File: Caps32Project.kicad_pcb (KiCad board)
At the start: 2 copper layers, 23.9 x 20.7 mm, 41 parts, among them J1 Sh 1.0, J2 Sh 1.0, J3 USB_C_Receptacle_PowerOnly_6P, Q1 AO3401A, Q2 MBT3904DW1, SW1 Reset, SW2 Boot, U1 AP2112K-3.3, U2 ESP32-WROOM-32U, U3 MCP73831-2-OT, U4 MPU-6050

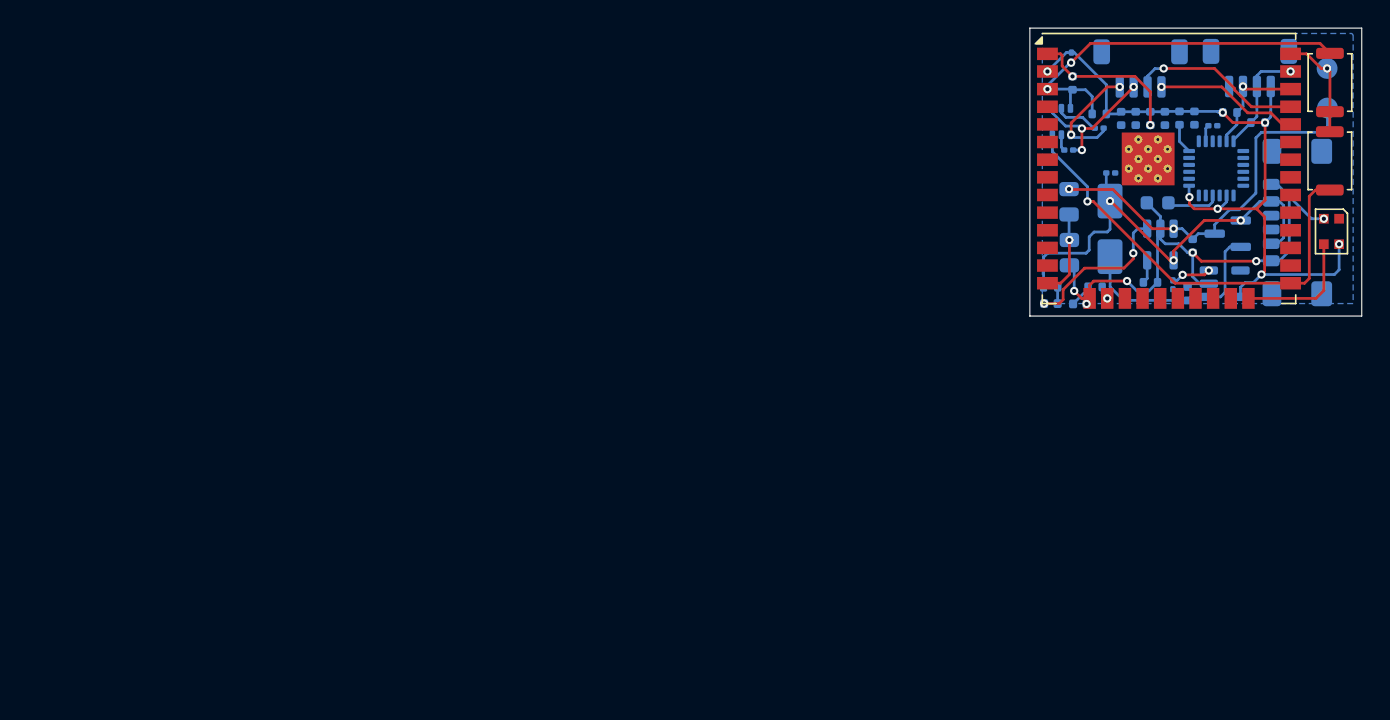
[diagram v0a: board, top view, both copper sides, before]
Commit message: Update Board
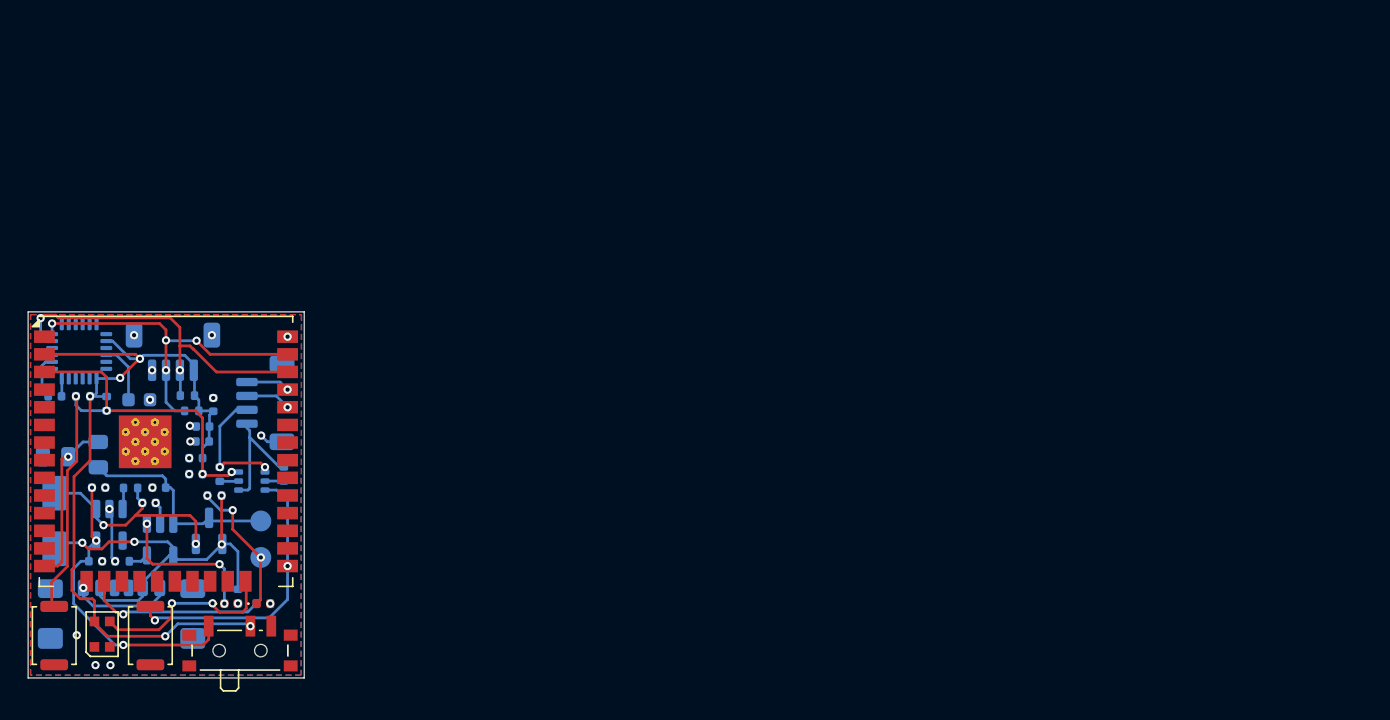
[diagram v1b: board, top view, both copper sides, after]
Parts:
- added SW3: SW_SPDT, Button_Switch_SMD:SW_SPDT_PCM12, F.Cu at (64.4, 82.3)
- C8: footprint Capacitor_SMD:C_0201_0603Metric -> Capacitor_SMD:C_0402_1005Metric
- D2, D4: moved to F.Cu
- J1, J2: value Sh 1.0 -> SH1.0
- R1, R2, R3, R4, R5: footprint Resistor_SMD:R_0201_0603Metric -> Resistor_SMD:R_0402_1005Metric
- moved SW1 100.1 mm to (51.0, 81.5)
- moved D5 93.1 mm to (54.5, 81.5), turned to 90 degrees
- moved SW2 91.5 mm to (57.9, 81.5), turned to 90 degrees
- moved J3 90.7 mm to (55.9, 81.2), turned to 180 degrees
- moved C8 85.6 mm to (51.0, 64.3)
- moved C3 85.3 mm to (54.0, 76.2), turned to 0 degrees
- moved TP2 84.4 mm to (65.9, 75.9), turned to -90 degrees
- moved U4 82.9 mm to (52.8, 61.1), turned to -90 degrees
- moved TP1 82.3 mm to (65.9, 73.3), turned to -90 degrees
- moved C2 82.2 mm to (54.2, 70.9), turned to 0 degrees
- moved U1 82.1 mm to (55.0, 73.6), turned to -90 degrees
- moved J2 80.2 mm to (59.5, 61.1)
- moved R10 79.5 mm to (60.6, 64.3)
- moved D1 78.8 mm to (51.0, 73.3), turned to -90 degrees
- moved R7 77.7 mm to (60.9, 65.4), turned to 180 degrees
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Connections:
- C2 pad 1: +3V3 -> Net-(SW3-A)
- C3 pad 1: +3V3 -> Net-(SW3-A)
- J1 pad 1: TX -> DTR
- J1 pad 2: RX -> RTS
- J1 pad 3: DTR -> TX
- J1 pad 4: RTS -> RX
- J1 pad MP: (no net) -> GND
- J2 pad 2: SDA -> SCL
- J2 pad 3: SCL -> SDA
- J2 pad MP: (no net) -> GND
- R10 pad 2: SDA -> SCL
- R7 pad 2: SCL -> SDA
- U1 pad 5: +3V3 -> Net-(SW3-A)
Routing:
- net GND: track 61.8 -> 25.8 mm, vias 9 -> 24
- net Net-(SW3-A): track 0.00 -> 21.6 mm, vias 0 -> 3
- net SCL: track 7.94 -> 26.2 mm, vias 1 -> 2
- net SDA: track 7.97 -> 25.1 mm, vias 1 -> 4
- net +BATT: track 27.5 -> 15.4 mm, vias 2 -> 0
- net LED: track 0.98 -> 13.0 mm
- net 0: track 32.0 -> 20.4 mm, vias 1 -> 2
- net EN: track 28.4 -> 39.9 mm, vias 2 -> 4
- net RX: track 12.5 -> 3.15 mm
- net +3V3: track 51.8 -> 59.1 mm, vias 7 -> 5
- net TX: track 10.4 -> 3.26 mm
- net SENSE: track 6.17 -> 11.9 mm
- net RGB_DI: track 9.00 -> 13.9 mm, vias 0 -> 2
- net VBUS: track 32.4 -> 29.4 mm, vias 3 -> 4
- net Net-(U4-CPOUT): track 1.20 -> 3.23 mm
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- added copper zone on F.Cu, net GND
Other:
- board size 23.9 x 20.7 mm -> 19.9 x 26.3 mm
